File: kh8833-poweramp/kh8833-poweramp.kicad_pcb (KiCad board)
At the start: 2 copper layers, 245 x 82 mm, 72 parts, among them J10 Conn_01x03, J11 Conn_01x03, J12 Conn_01x03, J7 Conn_01x03, J8 Conn_01x03, J9 Conn_01x06, U1 TDA2050, U2 TDA2050, U3 TDA2050, U4 TDA2050

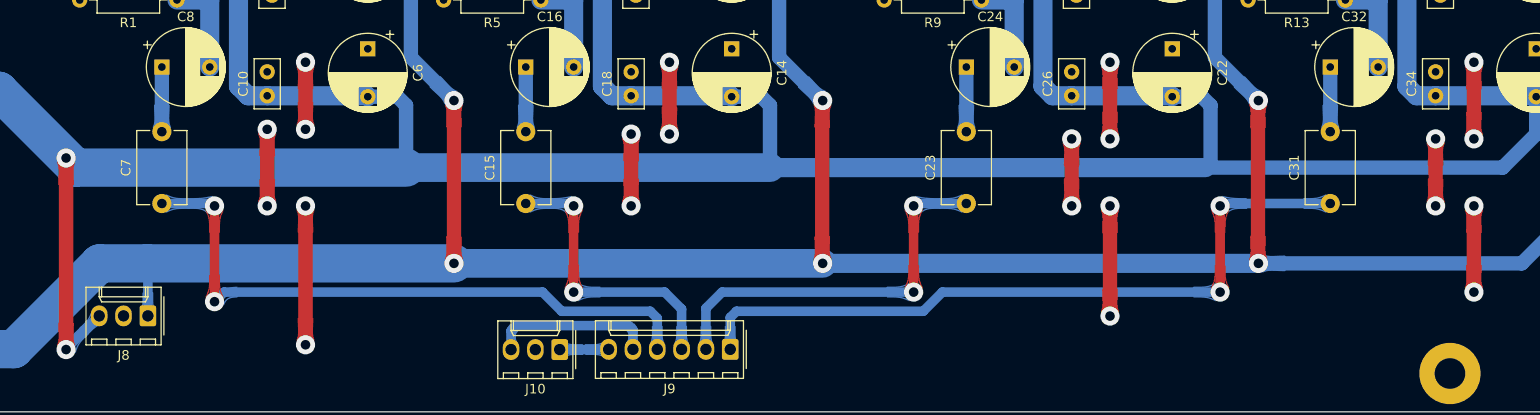
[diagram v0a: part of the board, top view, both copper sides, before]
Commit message: Add speaker protection
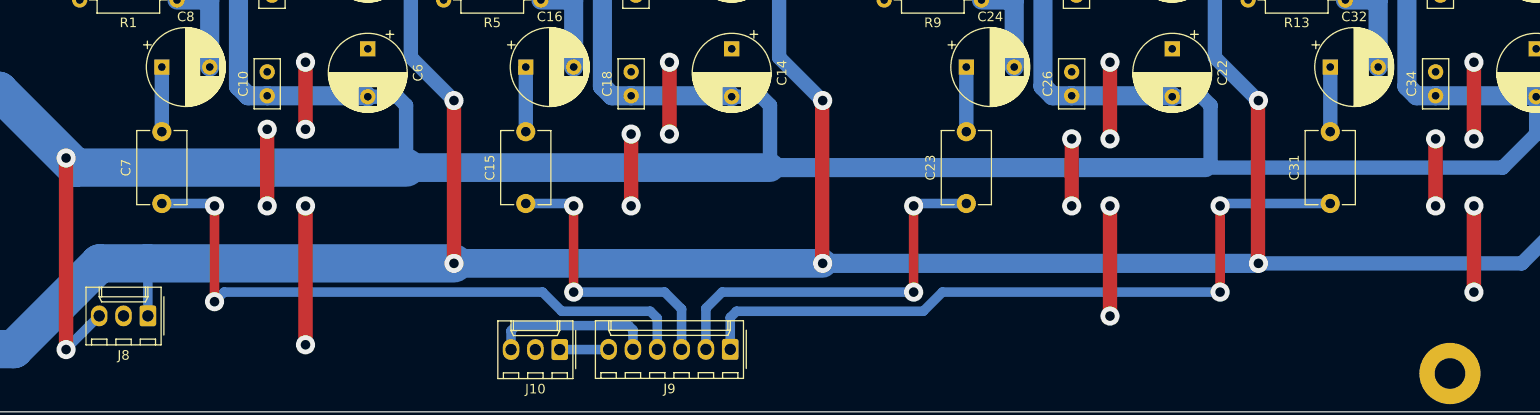
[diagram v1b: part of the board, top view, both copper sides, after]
